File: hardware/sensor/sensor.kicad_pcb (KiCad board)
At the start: 2 copper layers, 29 x 31 mm, 66 parts, among them P1 CONN_01X05, SW1 Reset, T1 BUK9Y22, T2 DMP10H4D2s, U1 LMR16006, U2 OPA376AIDCK, U3 CD74HC4046, U4 CD74HC4046, U5 Atmel_SAM_D09, U6 ZXGD3005E6_, X1 60V, X2 UART

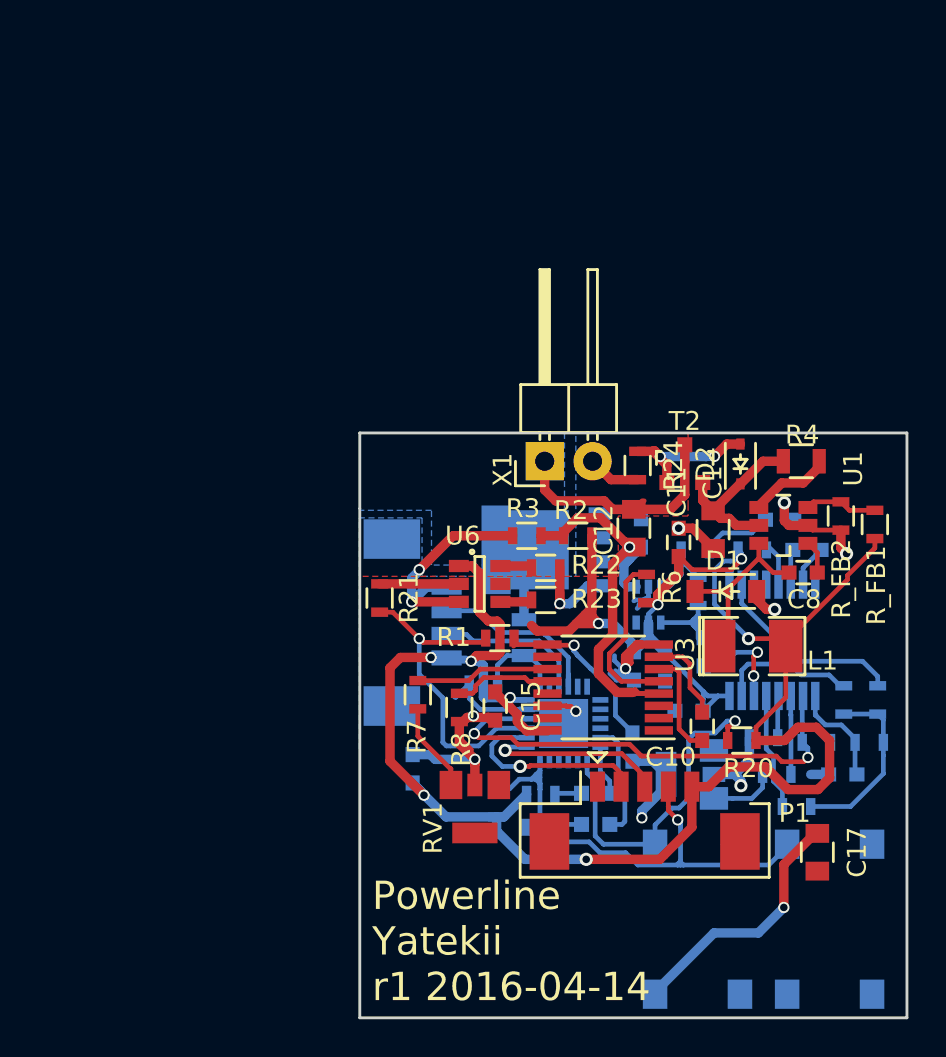
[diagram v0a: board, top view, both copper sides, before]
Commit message: PCB and schematic V2
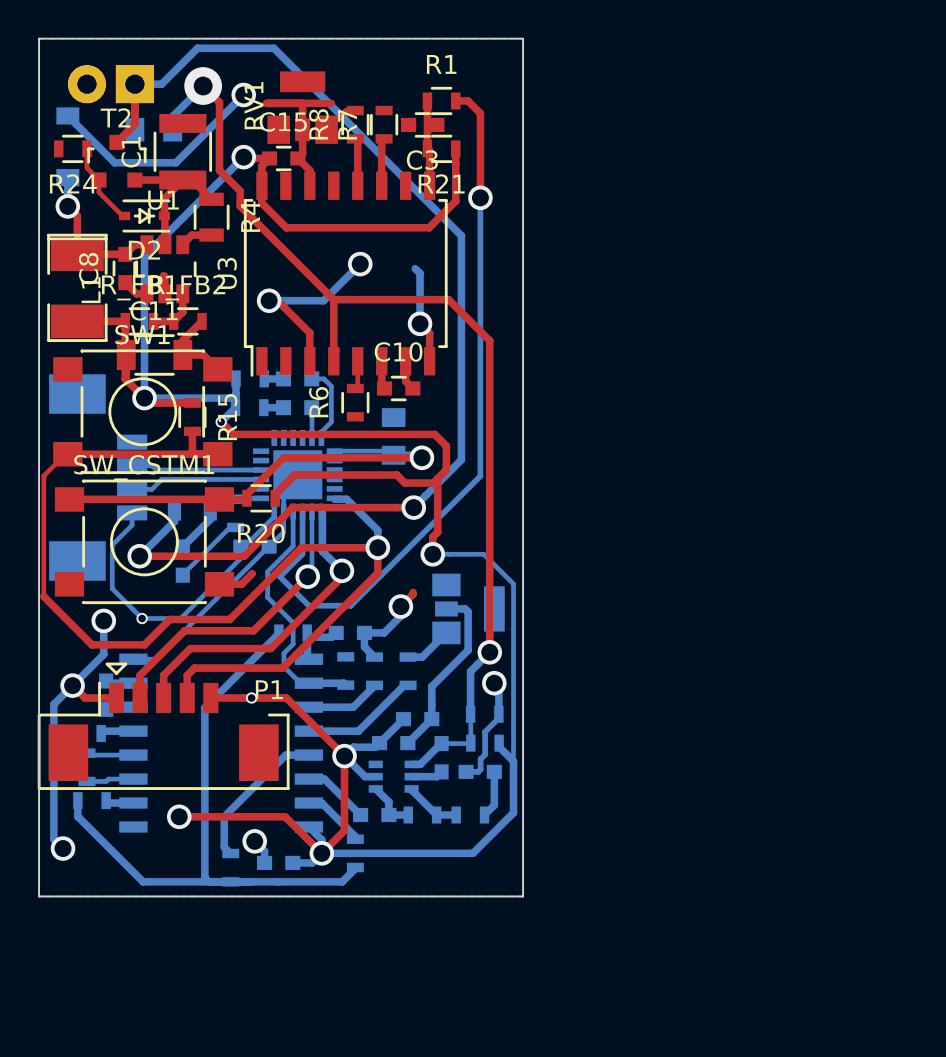
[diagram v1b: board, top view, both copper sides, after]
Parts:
- removed R22, R23: 0R, Resistors_SMD:R_0603
- removed T1: BUK9Y22, TO_SOT_Packages_SMD:SOT-669_LFPAK
- removed U6: ZXGD3005E6_, TO_SOT_Packages_SMD:SOT-23-6
- added C18: C_Small, Capacitors_SMD:C_0603, B.Cu at (134.6, 81.8)
- added JP3.4: R_Small, Resistors_SMD:R_0603, B.Cu at (129.5, 92.7)
- C1: footprint Capacitors_SMD:C_0805 -> Capacitors_SMD:C_1210
- C11: footprint Capacitors_SMD:C_0603 -> Capacitors_SMD:C_1206
- C12, C17, D1, R2, R3, X1: moved to B.Cu
- C3, R15, SW1, SW_CSTM1: moved to F.Cu
- D_BLUE1, D_RED1: footprint LEDs:LED-0603 -> LEDs:LED_0603
- P1: footprint Connectors_Molex:Connector_Molex_PicoBlade_53261-0571 -> Connectors_Molex:Molex_PicoBlade_53261-0571
- R1: value R_Small -> 10k
- R21: value 1k -> 100k
- U3, U4: footprint Housings_SSOP:TSSOP-16_4.4x5mm_Pitch0.65mm -> Housings_SOIC:SOIC-16_7.5x10.3mm_Pitch1.27mm
- X2: footprint Connectors_Molex:Connector_Molex_PicoBlade_53261-0471 -> Connectors_Molex:Molex_PicoBlade_53261-0471
- moved SW1 45.3 mm to (132.5, 73.9), turned to 0 degrees
- moved D1 42.1 mm to (128.5, 59.8), turned to 90 degrees
- moved JP3.1 42.0 mm to (129.8, 94.5), turned to 180 degrees
- moved L1 40.5 mm to (129.0, 67.3), turned to 270 degrees
- moved R_FB1 40.4 mm to (132.3, 69.1), turned to 0 degrees
- moved C8 39.4 mm to (131.6, 66.3), turned to 90 degrees
- moved RV1 38.4 mm to (141.0, 57.7), turned to 0 degrees
- moved C13 37.9 mm to (130.6, 88.9), turned to 90 degrees
- moved R11 36.6 mm to (129.5, 90.9), turned to 0 degrees
- moved R_FB2 36.1 mm to (134.9, 69.1), turned to 0 degrees
- moved SW_CSTM1 35.5 mm to (132.6, 80.8), turned to 0 degrees
- moved U1 35.5 mm to (133.7, 66.3), turned to 0 degrees
- moved C3 34.8 mm to (147.3, 58.7), turned to 180 degrees
- moved C1 34.5 mm to (134.6, 60.1), turned to 90 degrees
- moved R24 34.3 mm to (128.8, 59.9), turned to 180 degrees
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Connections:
- R11 pad 1: Net-(R11-Pad1) -> GND
- R11 pad 2: +3V3 -> Net-(R11-Pad2)
- R12 pad 2: Net-(R12-Pad2) -> GND
- R13 pad 2: GND -> Net-(R13-Pad2)
- R18 pad 1: Net-(R18-Pad1) -> +3V3
- R21 pad 1: /TX1_in -> +3V3
- R21 pad 2: Net-(R21-Pad2) -> Net-(C3-Pad1)
- R6 pad 1: +3V3 -> GND
- R7 pad 2: Net-(R7-Pad2) -> GND
- R8 pad 2: GND -> Net-(R8-Pad2)
- RV1 pad 3: Net-(R7-Pad2) -> Net-(R8-Pad2)
- RV1 pad 4: GND -> (no net)
- RV2 pad 1: Net-(RV2-Pad1) -> Net-(R13-Pad2)
- RV2 pad 3: Net-(R12-Pad2) -> Net-(RV2-Pad3)
- RV2 pad 4: GND -> (no net)
- U3 pad 3: Net-(U3-Pad3) -> GND
- U4 pad 4: /JP2 -> Net-(JP3.4-Pad1)
- U4 pad 5: Net-(R11-Pad1) -> Net-(R11-Pad2)
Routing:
- net VCC: track 16.8 -> 62.5 mm, vias 0 -> 2
- net GND: track 67.8 -> 101.4 mm, vias 12 -> 10
- net /coupling: track 23.0 -> 55.8 mm, vias 1 -> 2
- net Net-(P1-Pad4): track 27.6 -> 58.6 mm
- net +3V3: track 127.9 -> 157.8 mm
- net /VCOin: track 9.73 -> 34.5 mm
- net /TX1_in: track 17.4 -> 38.9 mm
- net /RX1_out: track 25.0 -> 13.2 mm, vias 2 -> 0
- net Net-(JP3.1-Pad1): track 10.3 -> 1.50 mm
- net Net-(R6-Pad2): track 9.14 -> 1.50 mm
- net /SW_CSTM: track 32.1 -> 24.5 mm, vias 2 -> 1
- net Net-(P1-Pad3): track 10.3 -> 16.7 mm
- net Net-(P1-Pad2): track 10.7 -> 15.8 mm
- net Net-(R22-Pad2): track 4.79 -> 0.00 mm, vias 1 -> 0
- net Net-(R7-Pad2): track 4.78 -> 0.00 mm
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- removed copper zone on B.Cu, net VCC
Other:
- board size 29 x 31 mm -> 25.7 x 45.5 mm
- net class pro4_default removed
- rule pad_to_mask_clearance: 0.2 -> 0
- rule trace_min: 0.2 -> 0.24
- rule via_min_size: 0.4 -> 0.9
- board text removed: "Powerline Yatekii r1 2016-04-14"
